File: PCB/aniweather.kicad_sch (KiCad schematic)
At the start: 34 parts, among them SW1 SW_DIP_x01, SW2 SW_Push, SW3 SW_Push, U5 TPS63001

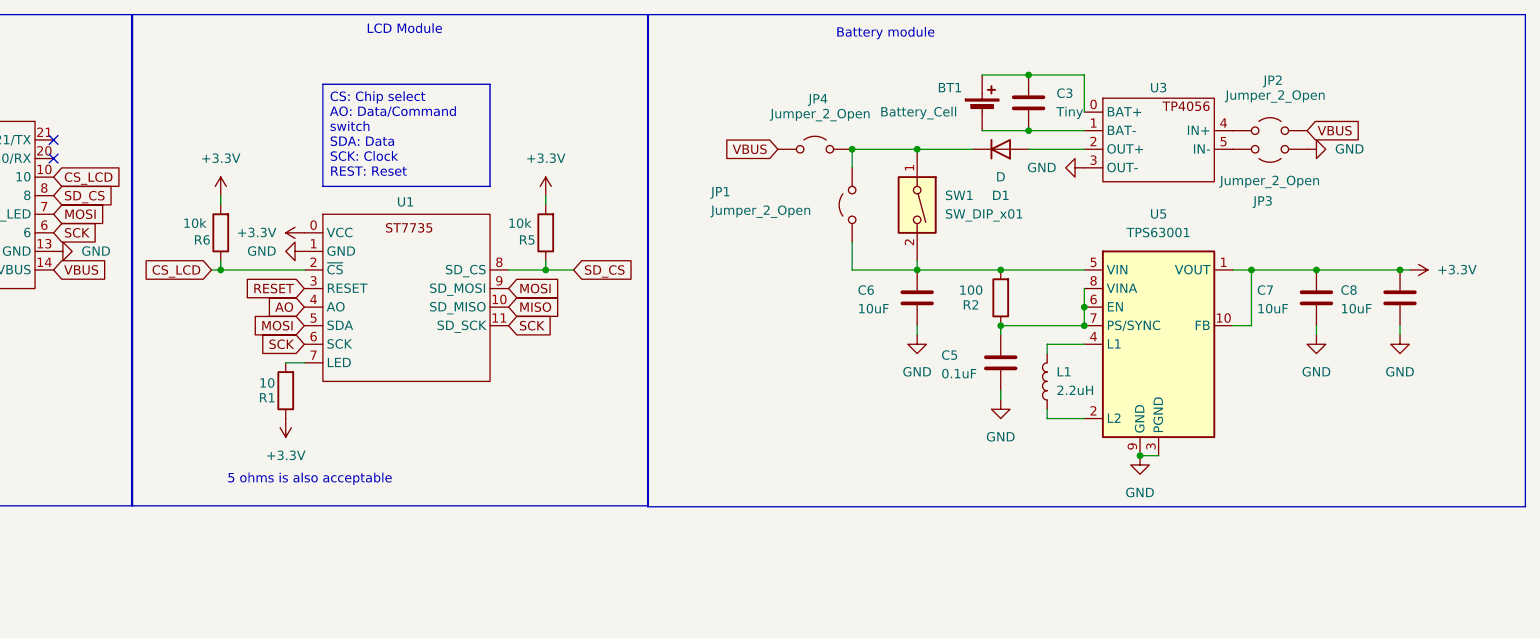
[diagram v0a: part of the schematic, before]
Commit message: Hope last rev
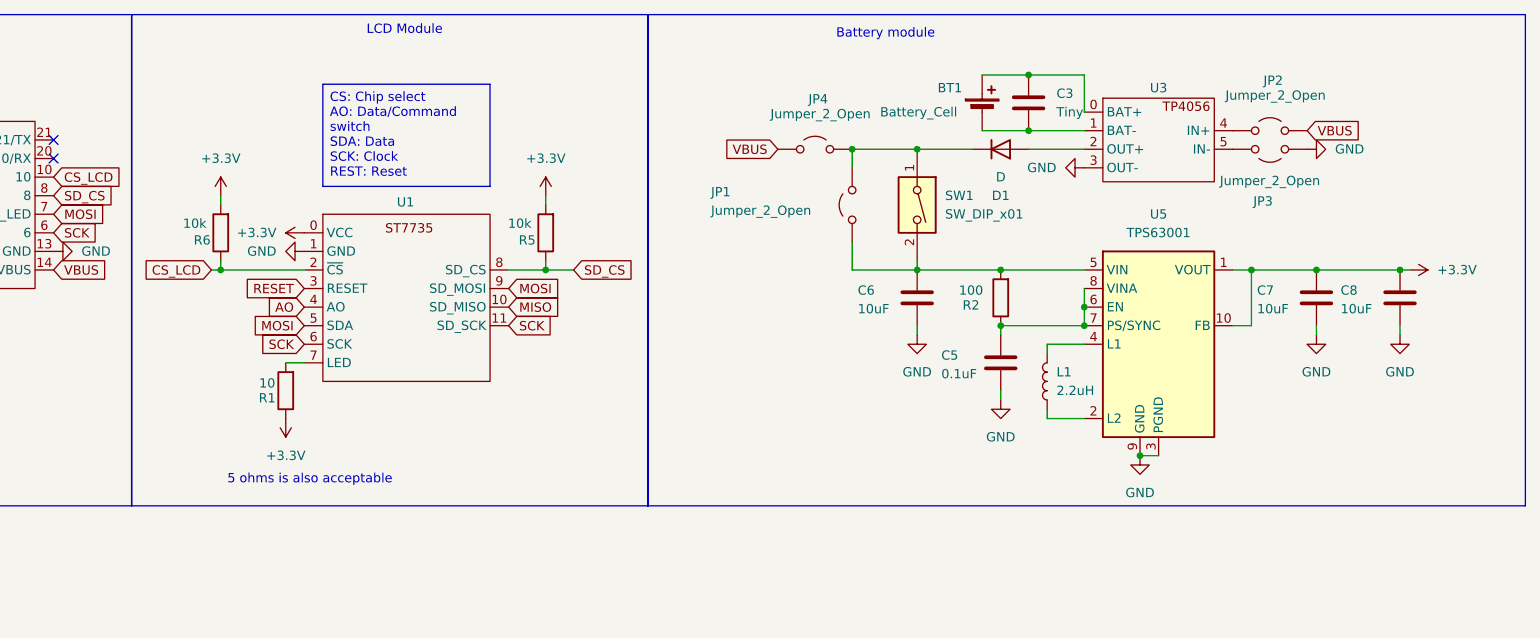
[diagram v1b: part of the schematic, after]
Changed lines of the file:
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@@
 	(rectangle
 		(start 165.1 12.065)
-		(end 285.115 79.375)
+		(end 285.115 79.248)
 		(stroke
 			(width 0)
@@
 	)
 	(rectangle
-		(start 94.615 12.065)
+		(start 94.488 12.065)
 		(end 165.1 79.248)
 		(stroke
